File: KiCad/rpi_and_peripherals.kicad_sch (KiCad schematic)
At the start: 5 parts, among them U3 PCM5102A, U4 PCM1808-Q1_PW_14

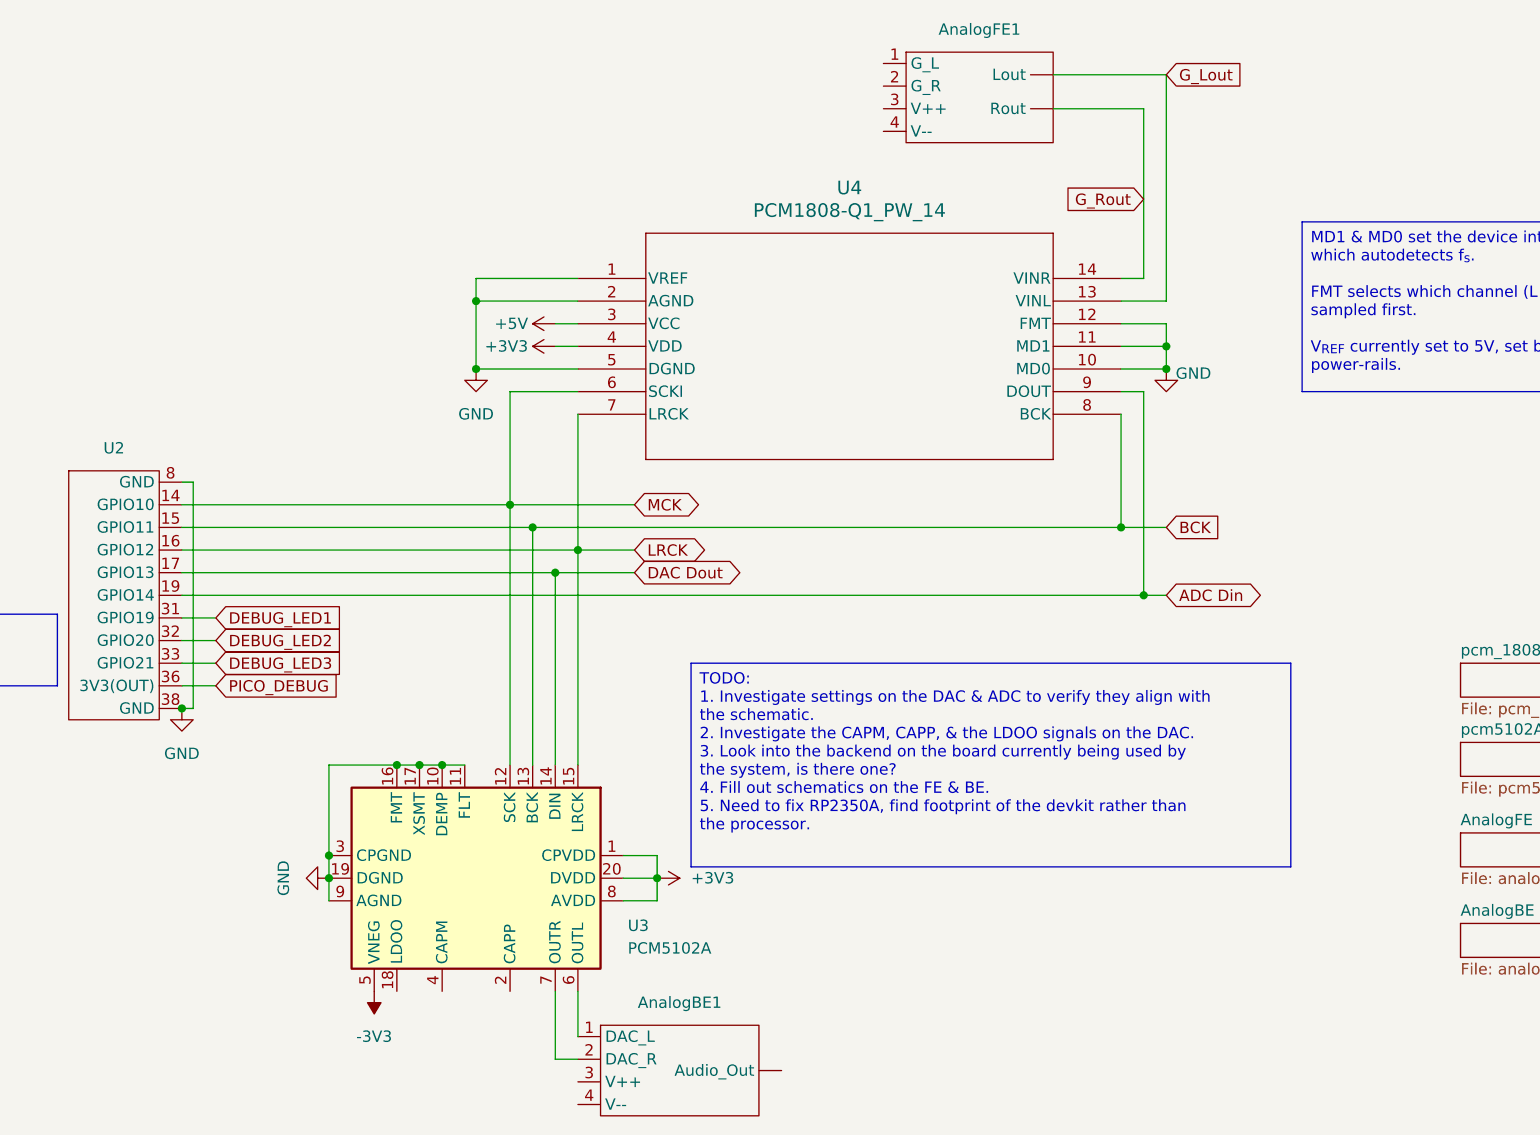
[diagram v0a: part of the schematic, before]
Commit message: Filled out FE schematic block
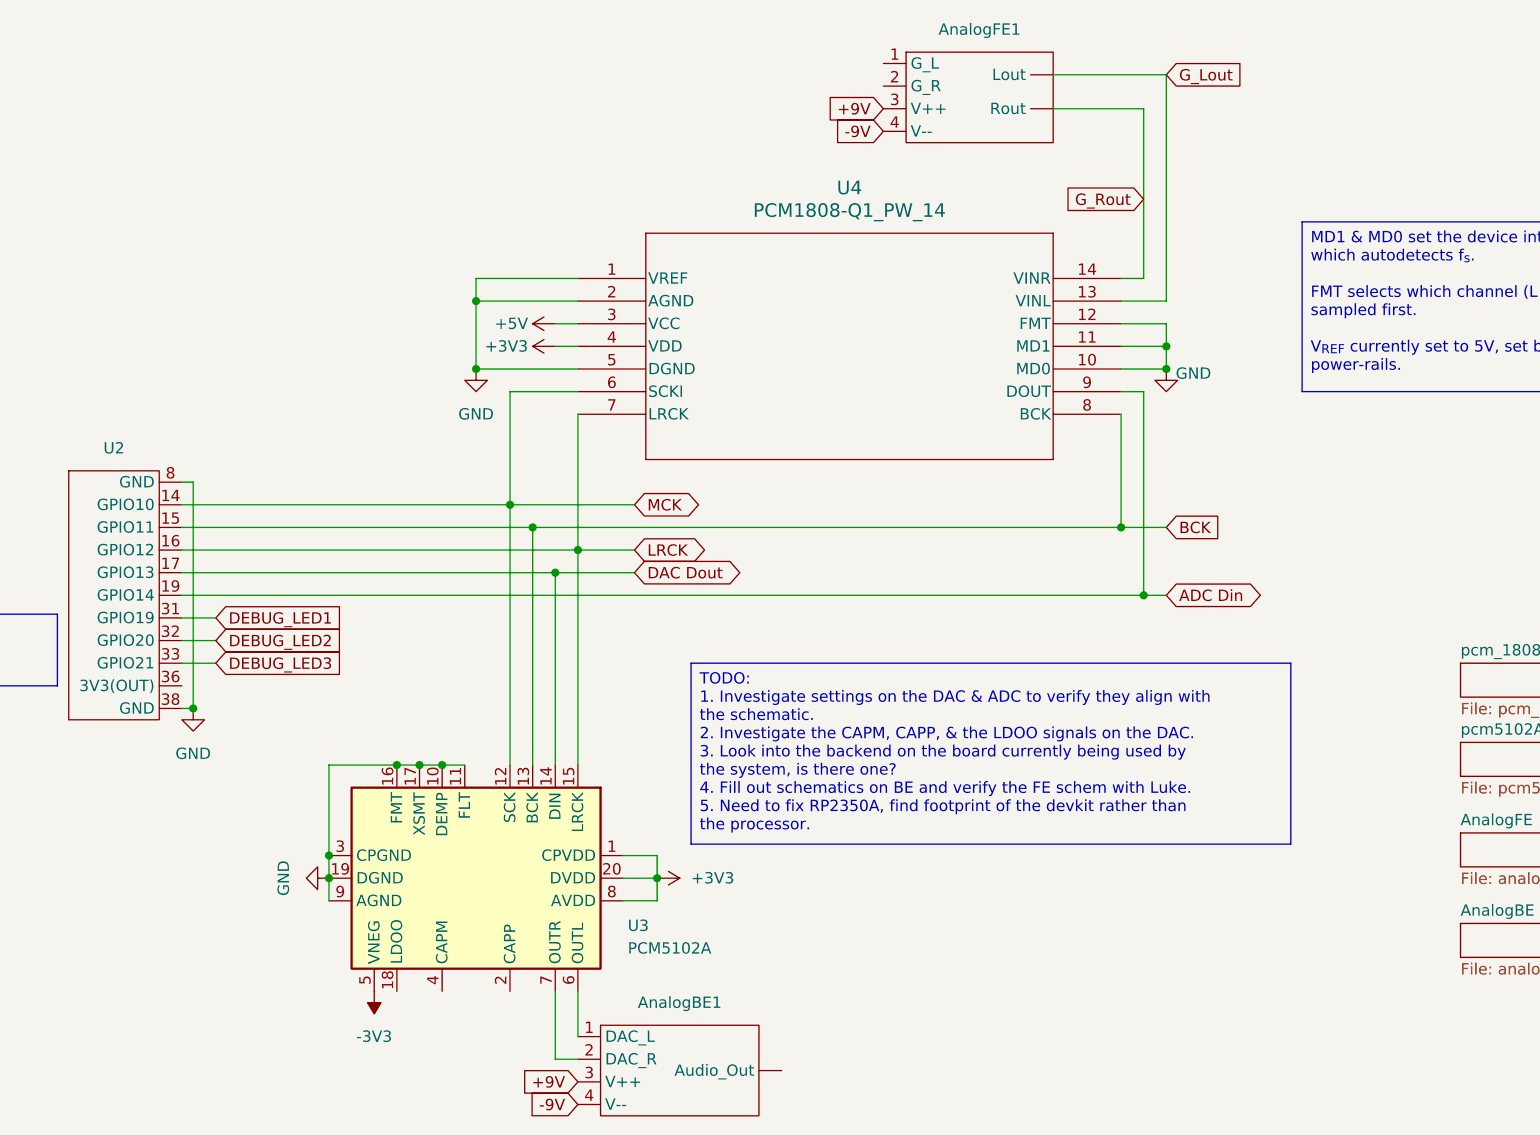
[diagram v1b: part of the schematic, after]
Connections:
- net +9V: now reaches AnalogFE1.3 (V++)
- net +9V: now also AnalogBE1.3 (V++)
- net -9V: now reaches AnalogFE1.4 (V--)
- net -9V: now also AnalogBE1.4 (V--)
- net PICO_DEBUG: no longer names the net of U2.36 (3V3(OUT))
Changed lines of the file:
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@@
 		)
 	)
-	(text_box "TODO:\n1. Investigate settings on the DAC & ADC to verify they align with the schematic.\n2. Investigate the CAPM, CAPP, & the LDOO signals on the DAC.\n3. Look into the backend on the board currently being used by the system, is there one?\n4. Fill out schematics on the FE & BE. \n5. Need to fix RP2350A, find footprint of the devkit rather than the processor. "
+	(text_box "TODO:\n1. Investigate settings on the DAC & ADC to verify they align with the schematic.\n2. Investigate the CAPM, CAPP, & the LDOO signals on the DAC.\n3. Look into the backend on the board currently being used by the system, is there one?\n4. Fill out schematics on BE and verify the FE schem with Luke.\n5. Need to fix RP2350A, find footprint of the devkit rather than the processor. "
 		(exclude_from_sim no)
 		(at 163.83 100.33 0)
-		(size 67.31 22.86)
+		(size 67.31 20.3053)
 		(margins 0.9525 0.9525 0.9525 0.9525)
 		(stroke
@@
 	)
 	(junction
+		(at 107.95 105.41)
+		(diameter 0)
+		(color 0 0 0 0)
+	)
+	(junction
 		(at 146.05 85.09)
 		(diameter 0)
@@
 	)
 	(junction
-		(at 106.68 105.41)
-		(diameter 0)
-		(color 0 0 0 0)
-	)
-	(junction
 		(at 212.09 85.09)
 		(diameter 0)
@@
 	(wire
 		(pts
-			(xy 106.68 105.41) (xy 107.95 105.41)
-		)
-		(stroke
-			(width 0)
-			(type default)
-		)
-	)
-	(wire
-		(pts
 			(xy 106.68 92.71) (xy 214.63 92.71)
 		)
@@
 	(wire
 		(pts
+			(xy 107.95 105.41) (xy 106.68 105.41)
+		)
+		(stroke
+			(width 0)
+			(type default)
+		)
+	)
+	(wire
+		(pts
 			(xy 204.47 34.29) (xy 217.17 34.29)
 		)
@@
 		(pts
 			(xy 151.13 87.63) (xy 106.68 87.63)
-		)
-		(stroke
-			(width 0)
-			(type default)
-		)
-	)
-	(wire
-		(pts
-			(xy 106.68 102.87) (xy 110.49 102.87)
 		)
 		(stroke
@@
 					(size 1.27 1.27)
 				)
+			)
+		)
+	)
+	(global_label "+9V"
+		(shape input)
+		(at 185.42 38.1 180)
+		(fields_autoplaced yes)
+		(effects
+			(font
+				(size 1.27 1.27)
+			)
+			(justify right)
+		)
+		(property "Intersheetrefs" "${INTERSHEET_REFS}"
+			(at 178.5643 38.1 0)
+			(hide yes)
+			(show_name no)
+			(do_not_autoplace no)
+			(effects
+				(font
+					(size 1.27 1.27)
+				)
+				(justify right)
 			)
 		)
@@
 		)
 	)
-	(global_label "PICO_DEBUG"
+	(global_label "+9V"
 		(shape input)
-		(at 110.49 102.87 0)
+		(at 151.13 147.32 180)
 		(fields_autoplaced yes)
 		(effects
@@
 				(size 1.27 1.27)
 			)
-			(justify left)
+			(justify right)
 		)
 		(property "Intersheetrefs" "${INTERSHEET_REFS}"
-			(at 125.2076 102.87 0)
-			(hide yes)
-			(show_name no)
-			(do_not_autoplace no)
-			(effects
-				(font
-					(size 1.27 1.27)
-				)
-				(justify left)
+			(at 144.2743 147.32 0)
+			(hide yes)
+			(show_name no)
+			(do_not_autoplace no)
+			(effects
+				(font
+					(size 1.27 1.27)
+				)
+				(justify right)
+			)
+		)
+	)
+	(global_label "-9V"
+		(shape input)
+		(at 151.13 149.86 180)
+		(fields_autoplaced yes)
+		(effects
+			(font
+				(size 1.27 1.27)
+			)
+			(justify right)
+		)
+		(property "Intersheetrefs" "${INTERSHEET_REFS}"
+			(at 144.2743 149.86 0)
+			(hide yes)
+			(show_name no)
+			(do_not_autoplace no)
+			(effects
+				(font
+					(size 1.27 1.27)
+				)
+				(justify right)
 			)
 		)
@@
 		(property "Intersheetrefs" "${INTERSHEET_REFS}"
 			(at 205.1135 48.26 0)
+			(hide yes)
+			(show_name no)
+			(do_not_autoplace no)
+			(effects
+				(font
+					(size 1.27 1.27)
+				)
+				(justify right)
+			)
+		)
+	)
+	(global_label "-9V"
+		(shape input)
+		(at 185.42 40.64 180)
+		(fields_autoplaced yes)
+		(effects
+			(font
+				(size 1.27 1.27)
+			)
+			(justify right)
+		)
+		(property "Intersheetrefs" "${INTERSHEET_REFS}"
+			(at 178.5643 40.64 0)
 			(hide yes)
 			(show_name no)
@@
 	(symbol
 		(lib_id "power:GND")
-		(at 106.68 105.41 0)
+		(at 107.95 105.41 0)
 		(unit 1)
 		(body_style 1)
@@
 		(fields_autoplaced yes)
 		(property "Reference" "#PWR015"
-			(at 106.68 111.76 0)
+			(at 107.95 111.76 0)
 			(hide yes)
 			(show_name no)
@@
 		)
 		(property "Value" "GND"
-			(at 106.68 110.49 0)
+			(at 107.95 110.49 0)
 			(show_name no)
 			(do_not_autoplace no)
@@
 		)
 		(property "Footprint" ""
-			(at 106.68 105.41 0)
+			(at 107.95 105.41 0)
 			(hide yes)
 			(show_name no)
@@
 		)
 		(property "Datasheet" ""
-			(at 106.68 105.41 0)
+			(at 107.95 105.41 0)
 			(hide yes)
 			(show_name no)
@@
 		)
 		(property "Description" "Power symbol creates a global label with name \"GND\" , ground"
-			(at 106.68 105.41 0)
-			(hide yes)
-			(show_name no)
+			(at 107.95 105.41 0)
+			(hide yes)
+			(show_name no)

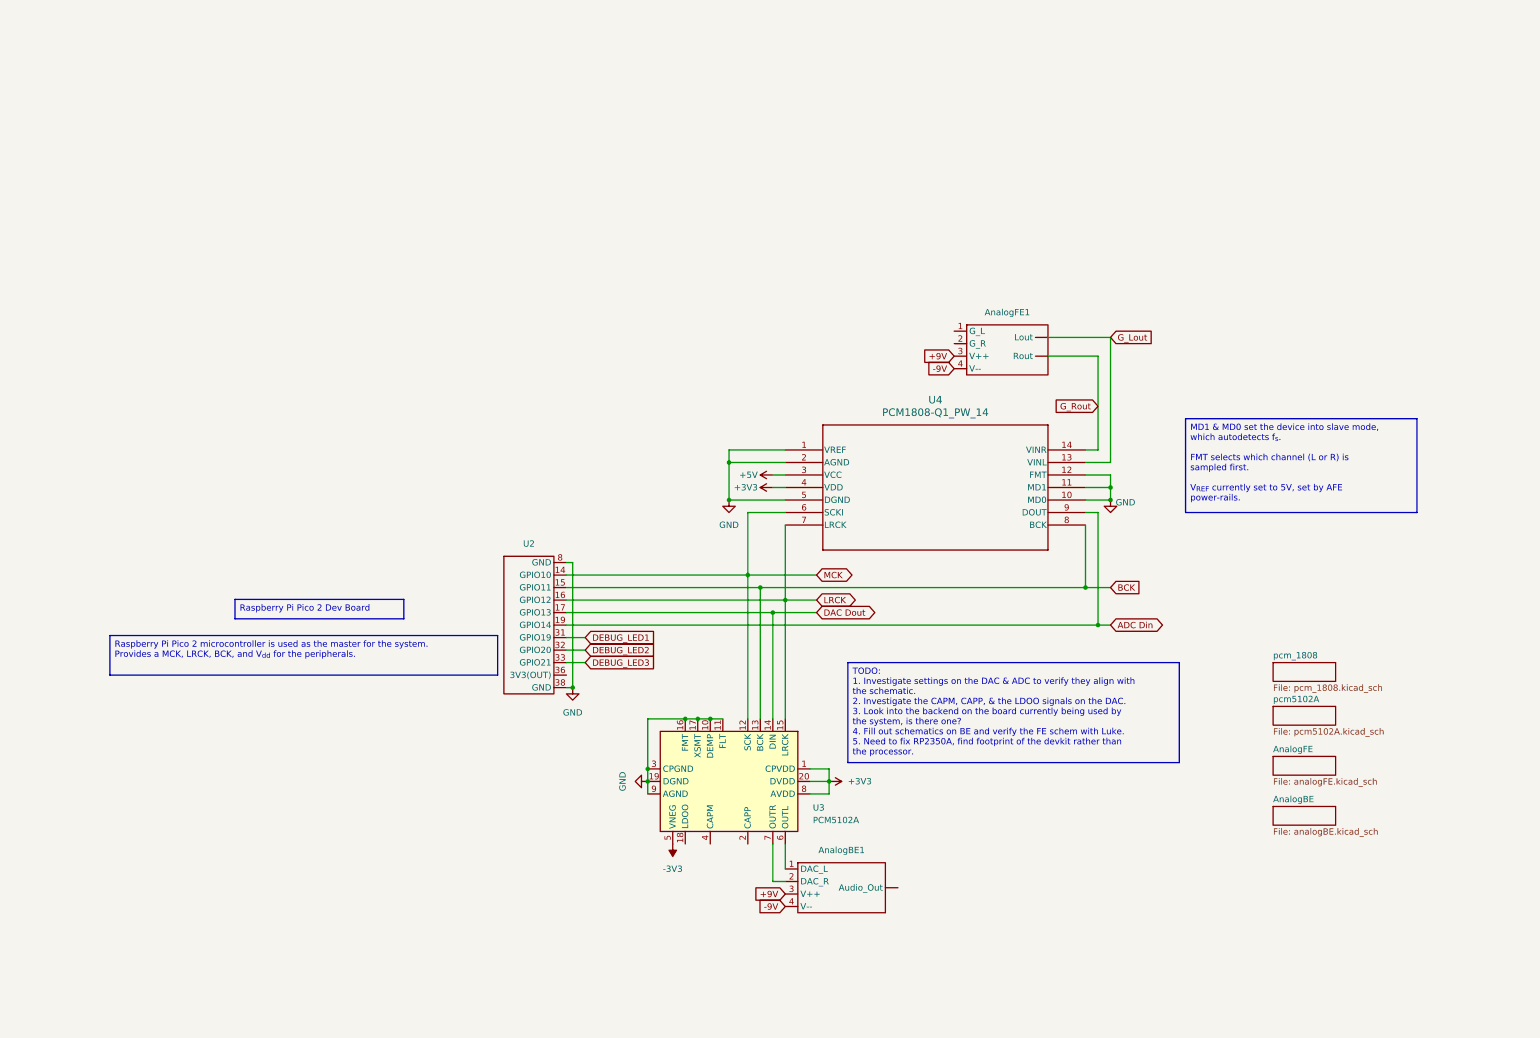
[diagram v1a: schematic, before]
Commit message: Changed footprints, added powersystem
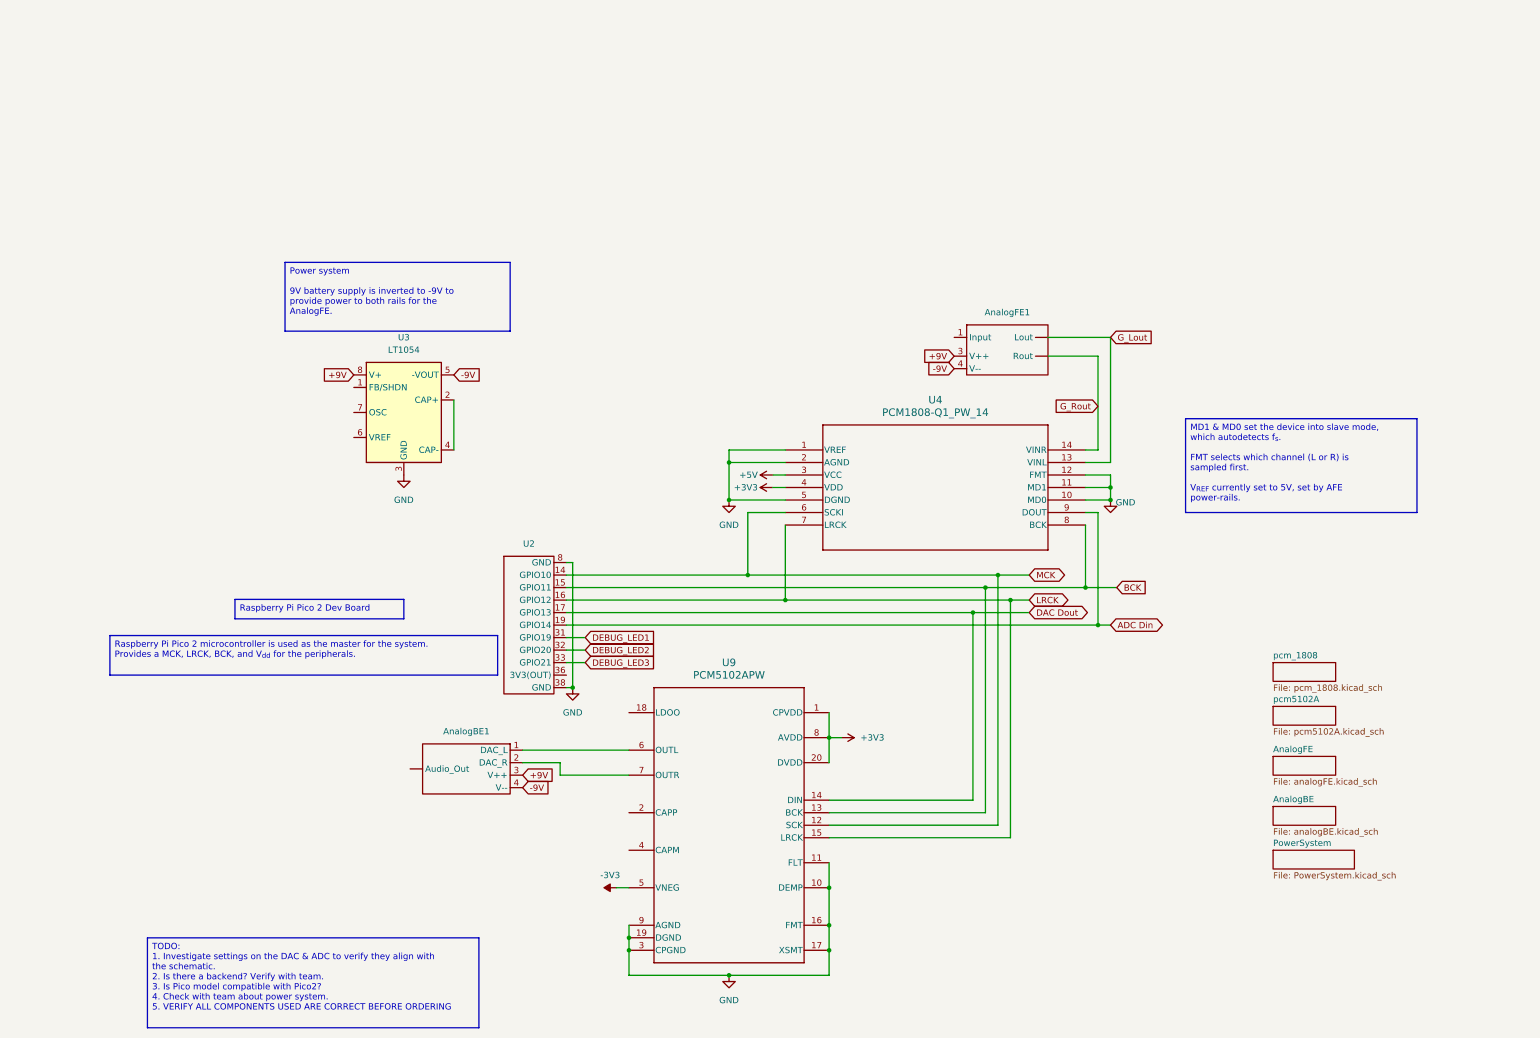
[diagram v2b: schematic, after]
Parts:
- removed U3: PCM5102A, Package_SO:TSSOP-20_4.4x6.5mm_P0.65mm, symbol Audio:PCM5102A
- added U3: LT1054, charge_pump:SOIC127P1030X265-16N, symbol Regulator_SwitchedCapacitor:LT1054
- added U9: PCM5102APW, Package_SO:Texas_PW0020A_TSSOP-20_4.4x6.5mm_P0.65mm, symbol DAC:PCM5102APW
- AnalogBE1, AnalogFE1: now in the parts list
- U2, U4: now left out of the parts list
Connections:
- net +3V3: now also U9.1 (CPVDD), U9.20 (DVDD), U9.8 (AVDD)
- net +9V: now also U3.8 (V+)
- net -3V3: now also U9.5 (VNEG)
- net -9V: now also U3.5 (-VOUT)
- net BCK: now also U9.13 (BCK)
- net DAC Dout: now also U9.14 (DIN)
- net GND: now also U3.3 (GND), U9.10 (DEMP), U9.11 (FLT), U9.16 (FMT), U9.17 (XSMT), U9.19 (DGND), U9.3 (CPGND), U9.9 (AGND)
- net LRCK: now also U9.15 (LRCK)
- net MCK: now also U9.12 (SCK)
- net at AnalogBE1.1 (DAC_L): now also U9.6 (OUTL)
- net at AnalogBE1.2 (DAC_R): now also U9.7 (OUTR)
- new net: U3.2 (CAP+), U3.4 (CAP-)
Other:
- added sheet PowerSystem (PowerSystem.kicad_sch)
- moved on the sheet: AnalogBE1
